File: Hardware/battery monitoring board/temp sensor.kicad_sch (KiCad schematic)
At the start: 11 parts, among them J2 Conn_01x02, U1 MAX31855KASA

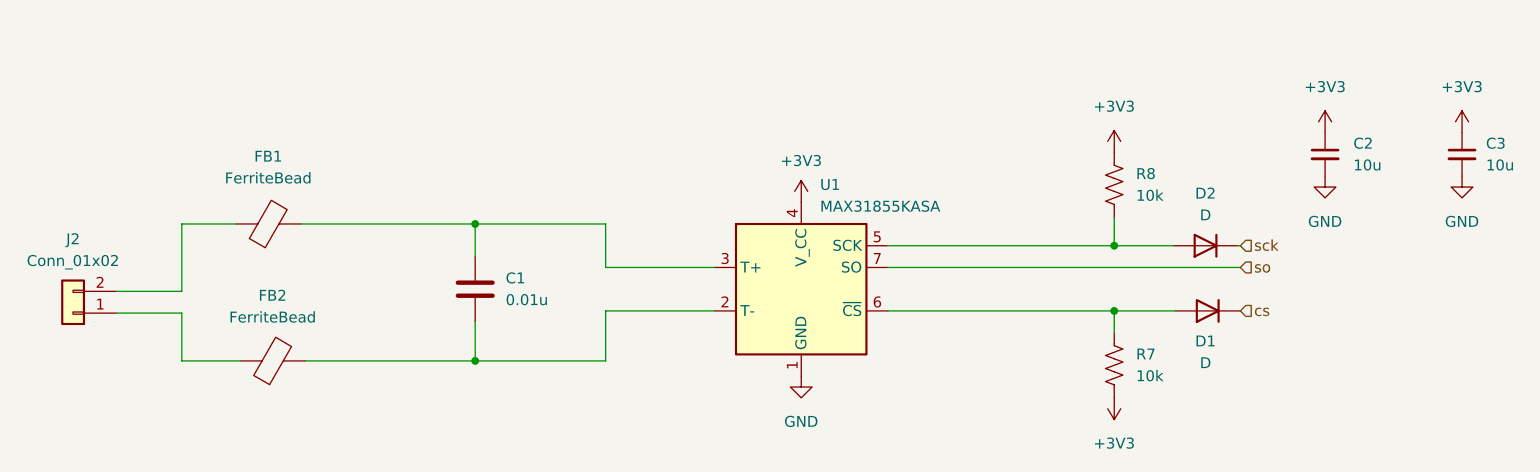
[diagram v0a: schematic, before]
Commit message: Revert "Merge branch 'hardware' of https://github.com/bruin-underwater-robotics/2023-2024 into hardware"
This reverts commit 1d5f0f31a35e539c7b0b2eac7ff2db3bf82506a7, reversing
changes made to b9b3862216192341382b87943b4a1d0c2c46b631.
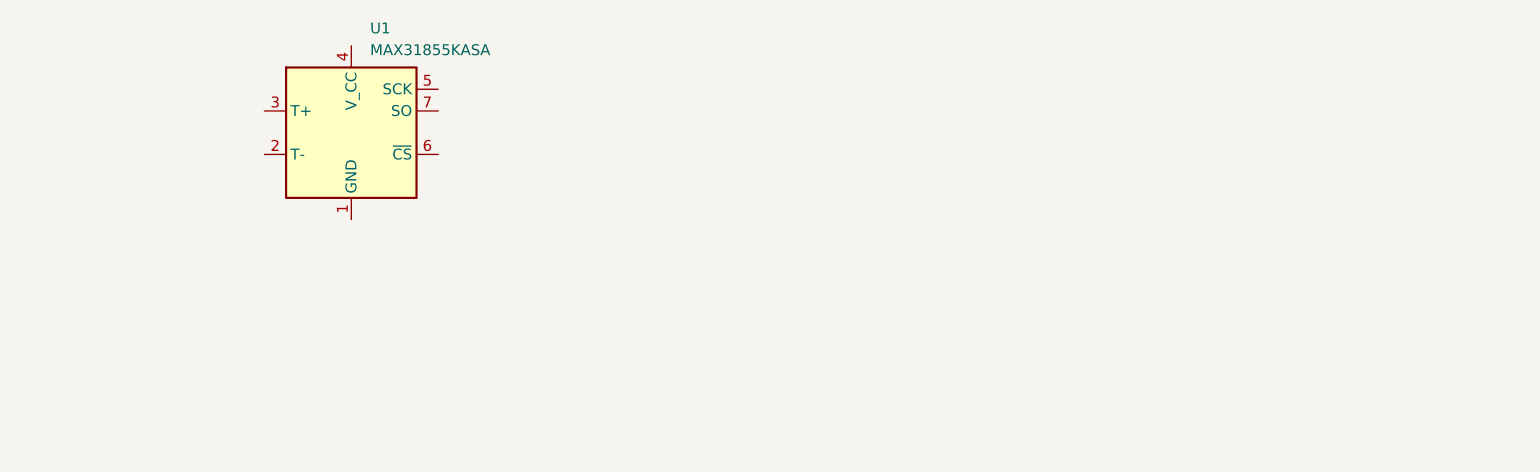
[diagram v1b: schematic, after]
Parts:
- removed C1: 0.01u, symbol Device:C
- removed C2, C3: 10u, symbol Device:C_Small
- removed D1, D2: D, symbol Device:D
- removed FB1, FB2: FerriteBead, symbol Device:FerriteBead
- removed J2: Conn_01x02, 4ms_Connector:Pins_1x02_2.54mm_TH, symbol PCM_4ms_Connector:Conn_01x02
- removed R7, R8: 10k, symbol Device:R_US
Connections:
- net +3V3: no longer names the net of U1.4 (V_CC)
- net GND: no longer names the net of U1.1 (GND)
- net so: no longer names the net of U1.7 (SO)
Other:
- moved on the sheet: U1
